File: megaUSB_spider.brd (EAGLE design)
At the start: 27.6 x 40.6 mm, 23 parts

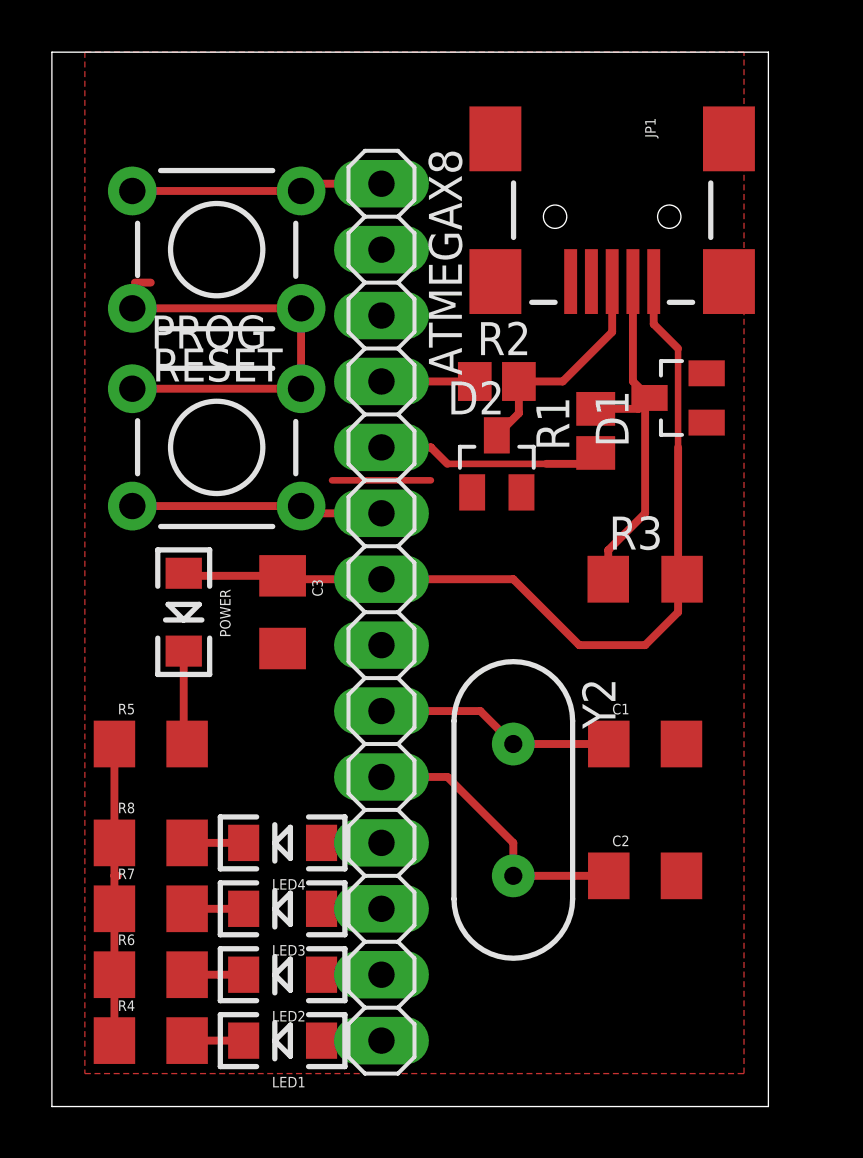
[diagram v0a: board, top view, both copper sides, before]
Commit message: cleanup of the old versions
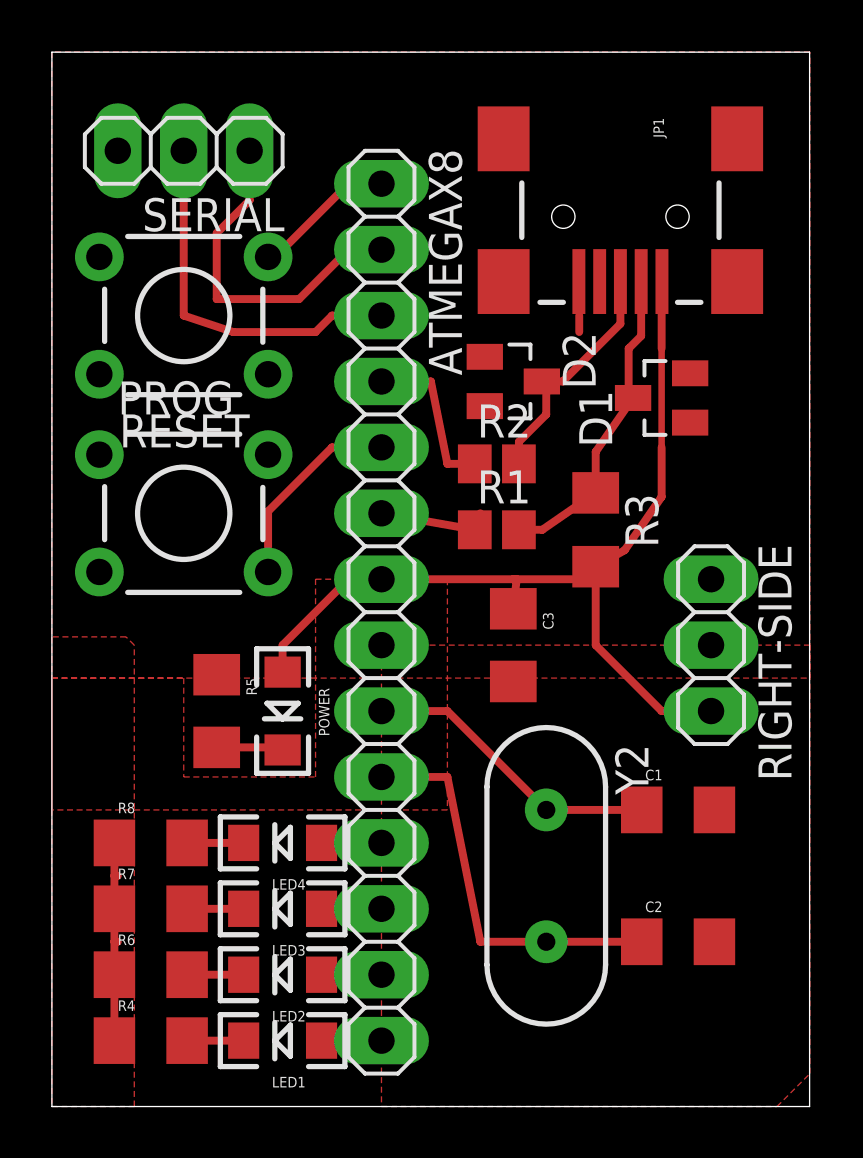
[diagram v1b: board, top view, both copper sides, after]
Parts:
- added RIGHT-SIDE, SERIAL: (no value), pinhead:1X03
- moved C3 8.98 mm to (76.2, 35.6)
- moved POWER 5.39 mm to (67.3, 33.0)
- moved R1 5.39 mm to (75.6, 40.0), turned to 0 degrees
- moved D2 3.24 mm to (76.2, 45.7), turned to 270 degrees
- moved R2 3.17 mm to (75.6, 42.5)
- moved C2 2.84 mm to (82.5, 24.1)
- moved R5 2.84 mm to (64.8, 33.0), turned to 270 degrees
- moved C1 2.84 mm to (82.5, 29.2)
- moved PROG 2.84 mm to (63.5, 40.6)
- moved RESET 2.84 mm to (63.5, 48.3)
- moved Y2 2.84 mm to (77.5, 26.7)
- moved R3 2.69 mm to (79.4, 40.0), turned to 270 degrees
- moved D1 0.63 mm to (81.9, 45.1)
- moved JP1 0.32 mm to (80.3, 52.1)
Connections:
- net GND: now also RIGHT-SIDE.1, SERIAL.3; no longer PROG.2, RESET.2
- net PD0: now also SERIAL.1
- net PD1: now also SERIAL.2
- net PROG: now also ATMEGAX8.5; no longer ATMEGAX8.6, PROG.3
- net RESET: no longer RESET.4
- net USBD-: now also ATMEGAX8.6; no longer ATMEGAX8.5
- net VCC: now also RIGHT-SIDE.3
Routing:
- net GND: track 32.7 -> 11.1 mm
- net PD1: track 0.00 -> 14.3 mm
- net PD0: track 0.00 -> 13.4 mm
- net USBD-: track 8.69 -> 4.32 mm
- net RESET: track 9.72 -> 5.49 mm
- net XTAL2: track 11.1 -> 15.2 mm
- net USBD+: track 3.59 -> 6.20 mm
- net VCC: track 34.0 -> 36.6 mm
- net D-: track 14.6 -> 12.3 mm
- net XTAL1: track 9.29 -> 11.6 mm
- net PROG: track 9.72 -> 7.73 mm
- net N$3: track 3.63 -> 2.58 mm
- net D+: track 8.76 -> 9.26 mm
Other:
- board size 27.6 x 40.6 mm -> 29.2 x 40.6 mm
